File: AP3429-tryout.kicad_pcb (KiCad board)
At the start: 2 copper layers, 90 x 50 mm, 31 parts, among them J1 Conn_01x05, J2 Conn_01x02, U1 AP3429, U2 AP3429, U3 AP3429, U4 AP2120N

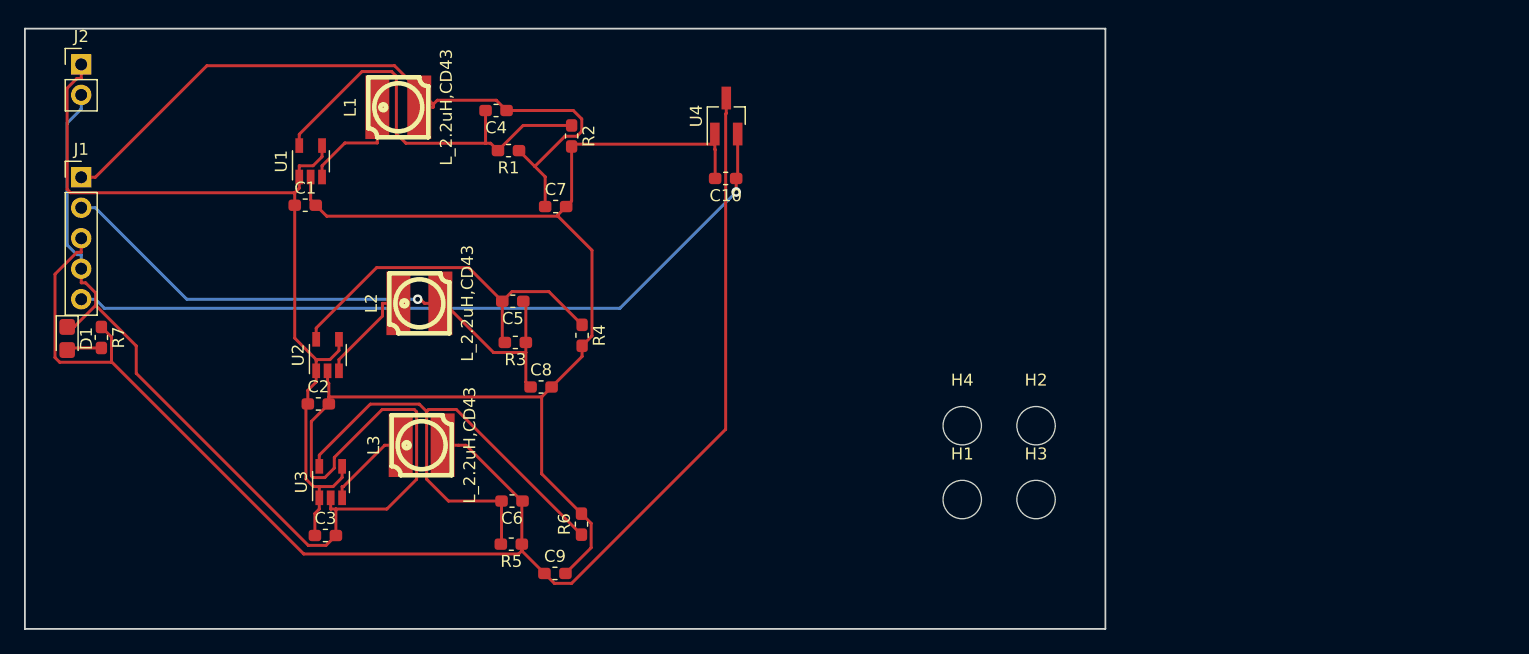
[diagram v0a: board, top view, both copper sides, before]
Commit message: update,
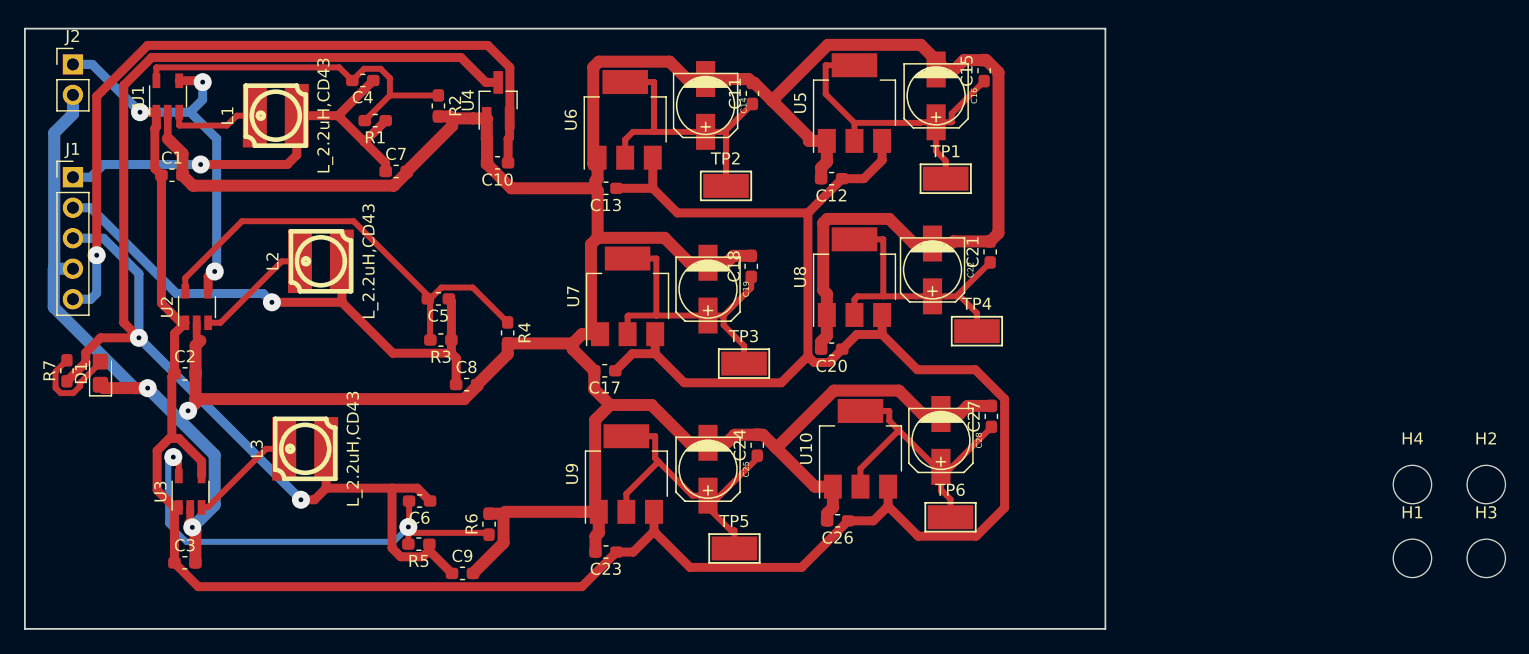
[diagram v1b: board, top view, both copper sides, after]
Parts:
- added C11: C104,0603, Capacitor_SMD:C_0603_1608Metric_Pad1.05x0.95mm_HandSolder, F.Cu at (60.6, 5.40)
- added C12: C104,0603, Capacitor_SMD:C_0603_1608Metric_Pad1.05x0.95mm_HandSolder, F.Cu at (67.2, 12.5)
- added C13: C104,0603, Capacitor_SMD:C_0603_1608Metric_Pad1.05x0.95mm_HandSolder, F.Cu at (48.4, 13.3)
- added C14: CP47uf,10V, w_smd_cap:c_elec_5x5.3, F.Cu at (56.7, 6.40)
- added C15: C104,0603, Capacitor_SMD:C_0603_1608Metric_Pad1.05x0.95mm_HandSolder, F.Cu at (79.9, 3.50)
- added C16: CP47uf,10V, w_smd_cap:c_elec_5x5.3, F.Cu at (75.9, 5.60)
- added C17: C104,0603, Capacitor_SMD:C_0603_1608Metric_Pad1.05x0.95mm_HandSolder, F.Cu at (48.3, 28.5)
- added C18: C104,0603, Capacitor_SMD:C_0603_1608Metric_Pad1.05x0.95mm_HandSolder, F.Cu at (60.5, 19.8)
- added C19: CP47uf,10V, w_smd_cap:c_elec_5x5.3, F.Cu at (56.9, 21.7)
- added C20: C104,0603, Capacitor_SMD:C_0603_1608Metric_Pad1.05x0.95mm_HandSolder, F.Cu at (67.2, 26.7)
- added C21: C104,0603, Capacitor_SMD:C_0603_1608Metric_Pad1.05x0.95mm_HandSolder, F.Cu at (80.4, 18.6)
- added C22: CP47uf,10V, w_smd_cap:c_elec_5x5.3, F.Cu at (75.6, 20.1)
- added C23: C104,0603, Capacitor_SMD:C_0603_1608Metric_Pad1.05x0.95mm_HandSolder, F.Cu at (48.4, 43.6)
- added C24: C104,0603, Capacitor_SMD:C_0603_1608Metric_Pad1.05x0.95mm_HandSolder, F.Cu at (61.0, 34.7)
- added C25: CP47uf,10V, w_smd_cap:c_elec_5x5.3, F.Cu at (56.9, 36.7)
- added C26: C104,0603, Capacitor_SMD:C_0603_1608Metric_Pad1.05x0.95mm_HandSolder, F.Cu at (67.7, 41.0)
- added C27: C104,0603, Capacitor_SMD:C_0603_1608Metric_Pad1.05x0.95mm_HandSolder, F.Cu at (80.5, 32.3)
- added C28: CP47uf,10V, w_smd_cap:c_elec_5x5.3, F.Cu at (76.3, 34.3)
- added TP1: TestPoint, TestPoint:TestPoint_Keystone_5019_Minature, F.Cu at (76.7, 12.5)
- added TP2: TestPoint, TestPoint:TestPoint_Keystone_5019_Minature, F.Cu at (58.4, 13.1)
- added TP3: TestPoint, TestPoint:TestPoint_Keystone_5019_Minature, F.Cu at (59.9, 27.9)
- added TP4: TestPoint, TestPoint:TestPoint_Keystone_5019_Minature, F.Cu at (79.3, 25.2)
- added TP5: TestPoint, TestPoint:TestPoint_Keystone_5019_Minature, F.Cu at (59.1, 43.3)
- added TP6: TestPoint, TestPoint:TestPoint_Keystone_5019_Minature, F.Cu at (77.1, 40.7)
- added U10: AMS1117-3.3, Package_TO_SOT_SMD:SOT-223-3_TabPin2, F.Cu at (69.6, 35.0)
- added U5: AMS1117-3.3, Package_TO_SOT_SMD:SOT-223-3_TabPin2, F.Cu at (69.1, 6.20)
- added U6: AMS1117-3.3, Package_TO_SOT_SMD:SOT-223-3_TabPin2, F.Cu at (50.0, 7.60)
- added U7: AMS1117-3.3, Package_TO_SOT_SMD:SOT-223-3_TabPin2, F.Cu at (50.2, 22.3)
- added U8: AMS1117-3.3, Package_TO_SOT_SMD:SOT-223-3_TabPin2, F.Cu at (69.1, 20.7)
- added U9: AMS1117-3.3, Package_TO_SOT_SMD:SOT-223-3_TabPin2, F.Cu at (50.1, 37.1)
- moved H1 37.8 mm to (115.6, 44.1)
- moved H2 37.8 mm to (121.7, 38.0)
- moved H3 37.8 mm to (121.7, 44.1)
- moved H4 37.8 mm to (115.6, 38.0)
- moved C10 19.0 mm to (39.4, 11.2)
- moved U4 19.0 mm to (39.4, 5.98)
- moved C7 13.6 mm to (30.9, 11.9)
- moved U1 13.1 mm to (11.9, 5.65)
- moved C3 11.9 mm to (13.3, 44.5)
- moved U3 11.7 mm to (13.8, 38.6)
- moved U2 11.6 mm to (14.3, 23.2)
- moved C1 11.4 mm to (12.2, 12.2)
- moved C2 11.4 mm to (13.3, 28.8)
- moved R1 11.4 mm to (29.2, 7.66)
- moved R2 11.4 mm to (34.4, 6.44)
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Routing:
- net +5V: track 72.6 -> 251.3 mm, vias 0 -> 3
- net GND: track 188.7 -> 355.9 mm, vias 0 -> 3
- net Net-(C15-Pad1): track 0.00 -> 27.4 mm
- net Net-(C24-Pad1): track 0.00 -> 26.7 mm
- net Net-(C27-Pad1): track 0.00 -> 25.9 mm
- net Net-(C18-Pad1): track 0.00 -> 25.6 mm
- net Net-(C21-Pad1): track 0.00 -> 24.7 mm
- net Net-(C11-Pad1): track 0.00 -> 24.5 mm
- net +1V2: track 60.8 -> 39.1 mm, vias 0 -> 1
- net Net-(C5-Pad2): track 31.3 -> 37.8 mm
- net Net-(C6-Pad2): track 45.4 -> 39.0 mm, vias 0 -> 2
- net Net-(D1-Pad2): track 2.92 -> 7.91 mm
- net Net-(C4-Pad2): track 34.9 -> 30.2 mm
- net +3V3: track 123.9 -> 120.4 mm, vias 0 -> 2
- net +1V8: track 49.4 -> 47.3 mm
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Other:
- net class Default: trace_width 0.25 -> 0.5; via_dia 0.8 -> 1.5
- net class GND added: clearance 0.2, trace_width 1, via_dia 1.5, via_drill 0.4
- net class PWR added: clearance 0.2, trace_width 0.75, via_dia 1.5, via_drill 0.4
